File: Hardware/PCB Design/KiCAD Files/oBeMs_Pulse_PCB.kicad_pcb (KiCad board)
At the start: 2 copper layers, 180.3 x 120.7 mm, 132 parts, among them P1 1WIRE, P10 5V, P11 3V3, P12 GND, P13 ADC_0-7, P14 ADC_8-15, P15 ADC_VREF_2, P16 ADC_VREF_1, P17 SPI_ADC_DAC, P18 DIO_OUTPUT, P19 PULL_UP, P2 EXT_CAP, P20 GROUND, P21 DIO_INPUT, P22 DIO_OUTPUT, P23 PULL_UP, P24 GROUND, P25 DIO_INPUT, P26 DIO_OUTPUT, P27 PULL_UP, P28 GROUND, P29 DIO_INPUT, P3 HARD_WDT, P34 DAC, P36 PROTOTYPING_AREA, P4 LED 5-8, P6 AC_INPUT, P7 LED 1-4, P8 LT_PWR, P9 V?, Q1 BC546, Q2 BC556, U1 LM2575, U2 DS18B20, U3 TLC555, U4 4017, U5 MCP3008, U6 MCP3008, U7 MCP4802, U8 LM2576

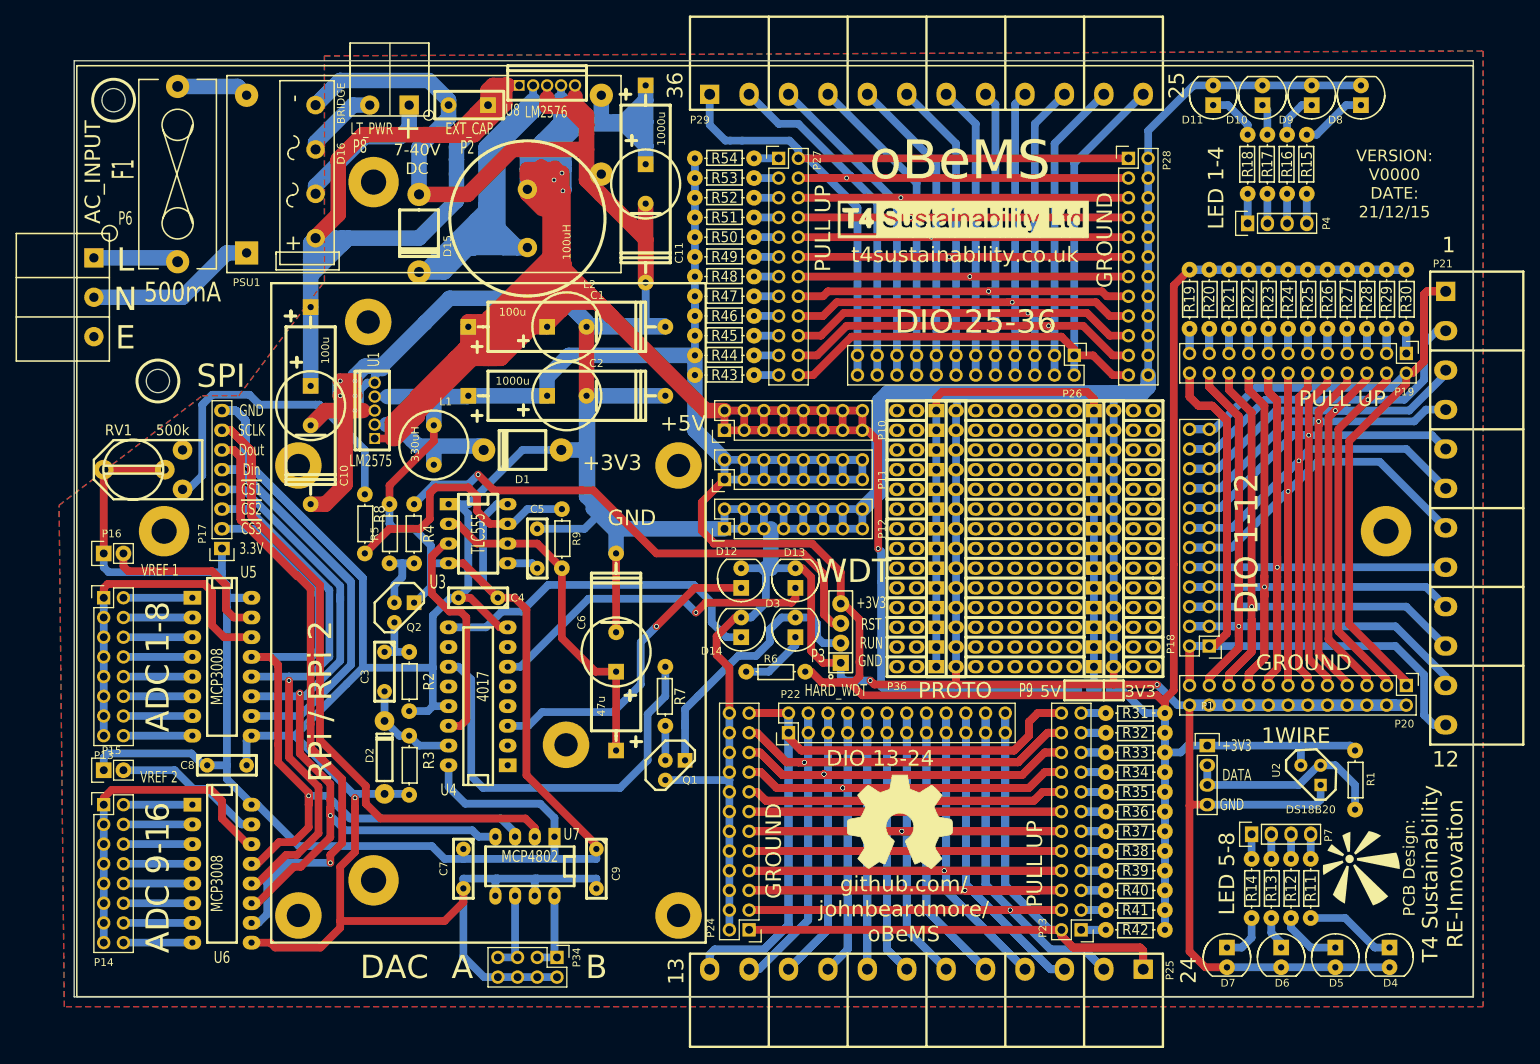
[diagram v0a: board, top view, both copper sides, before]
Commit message: Rev 6. Final changes before PCB v0000 done
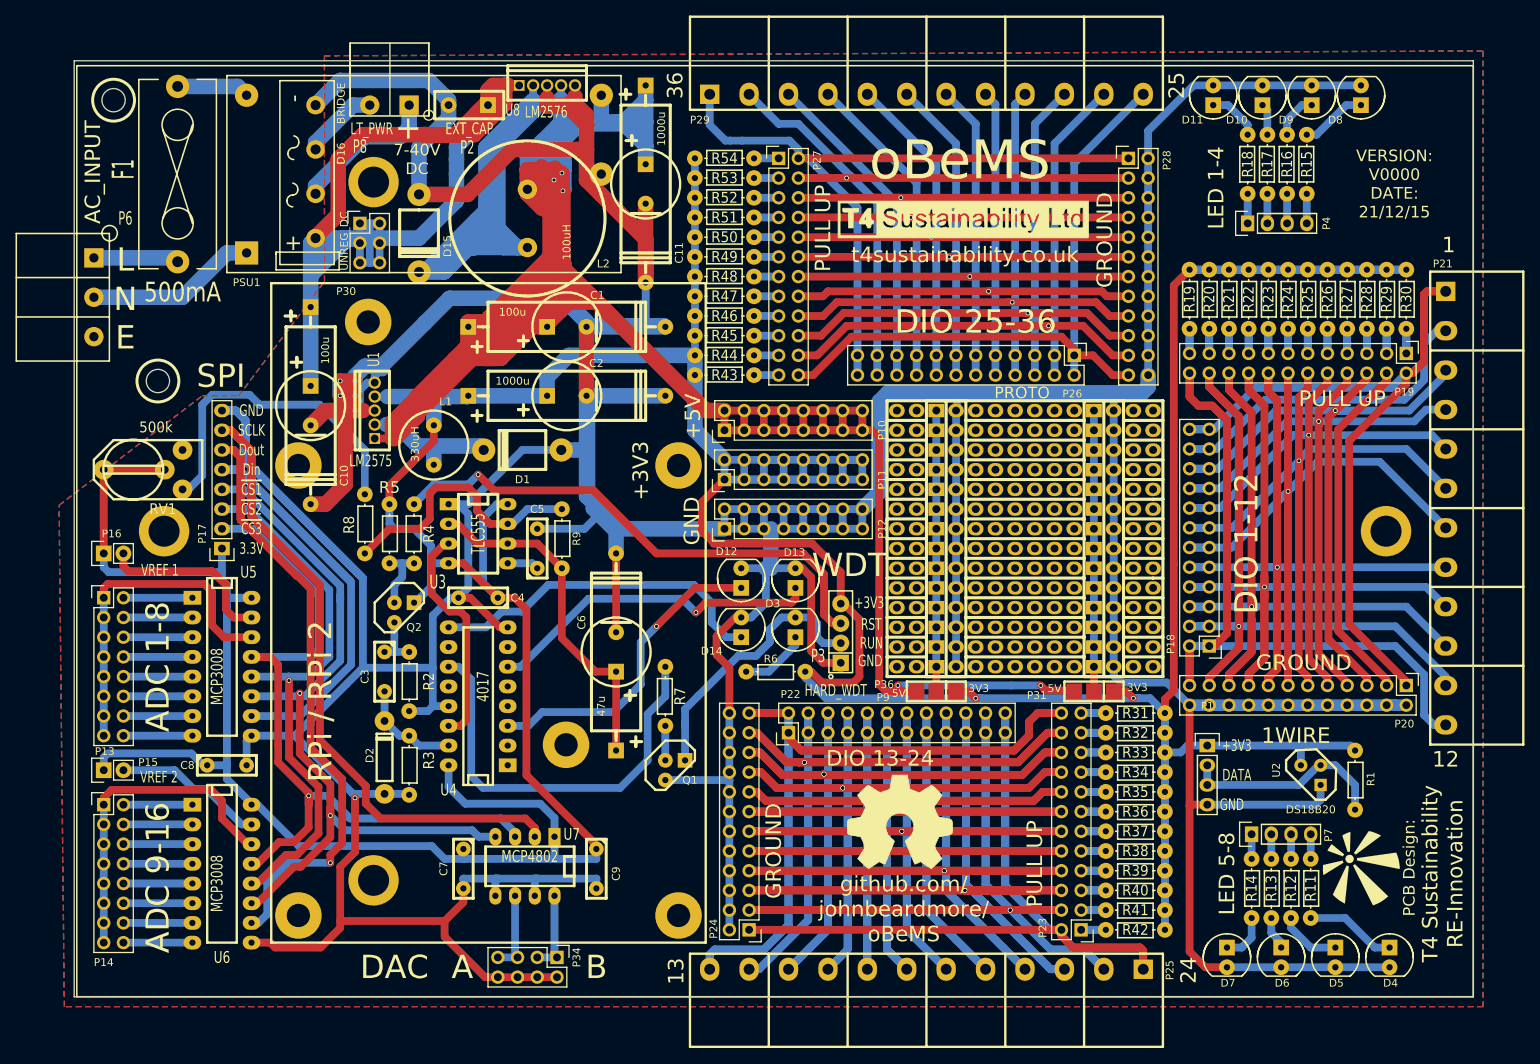
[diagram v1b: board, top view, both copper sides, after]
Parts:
- added P30: UNREG_DC, REInnovationFootprint:Pin_Header_Straight_2x03, F.Cu at (109.2, 56.5)
- added P31: V2?, REInnovationFootprint:SIL-3_solder_connect, F.Cu at (203.8, 116.8)
- H1, H2: value Bolt Hole -> AC Cover Mount Hole
- P36: footprint PROTO_AREA_16x14 -> REInnovationFootprint:PROTO_AREA_16x14
- P9: value V? -> V1?; footprint matts_components:SIL-3_solder_connect -> REInnovationFootprint:SIL-3_solder_connect
- PCB1: footprint REInnovationFootprint:PCB_120x150_WISKA -> PCB_120x150_WISKA
- RV1: footprint RV_various_lg_pad -> matts_components:RV_various_lg_pad
- moved P9 20.3 mm to (183.5, 116.8)
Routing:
- net Net-(P36-Pad1): track 93.3 -> 36.2 mm
- net GND: track 1161.5 -> 1117.1 mm, vias 8 -> 6
- net Net-(P31-Pad2): track 0.00 -> 36.2 mm
- net Net-(C10-Pad1): track 169.7 -> 196.0 mm
- net +5V: track 526.3 -> 530.8 mm, vias 4 -> 5
- net +3.3V: track 739.1 -> 742.2 mm, vias 0 -> 2
